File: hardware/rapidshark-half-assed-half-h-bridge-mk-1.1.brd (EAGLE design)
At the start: 17.8 x 33 mm, 29 parts, among them Q1 SPD15P10PL, Q2 IRLR3410, Q3 MMBT2222A, Q4 MMBT4403, U1 ARDUINO_PRO_MINIMINE

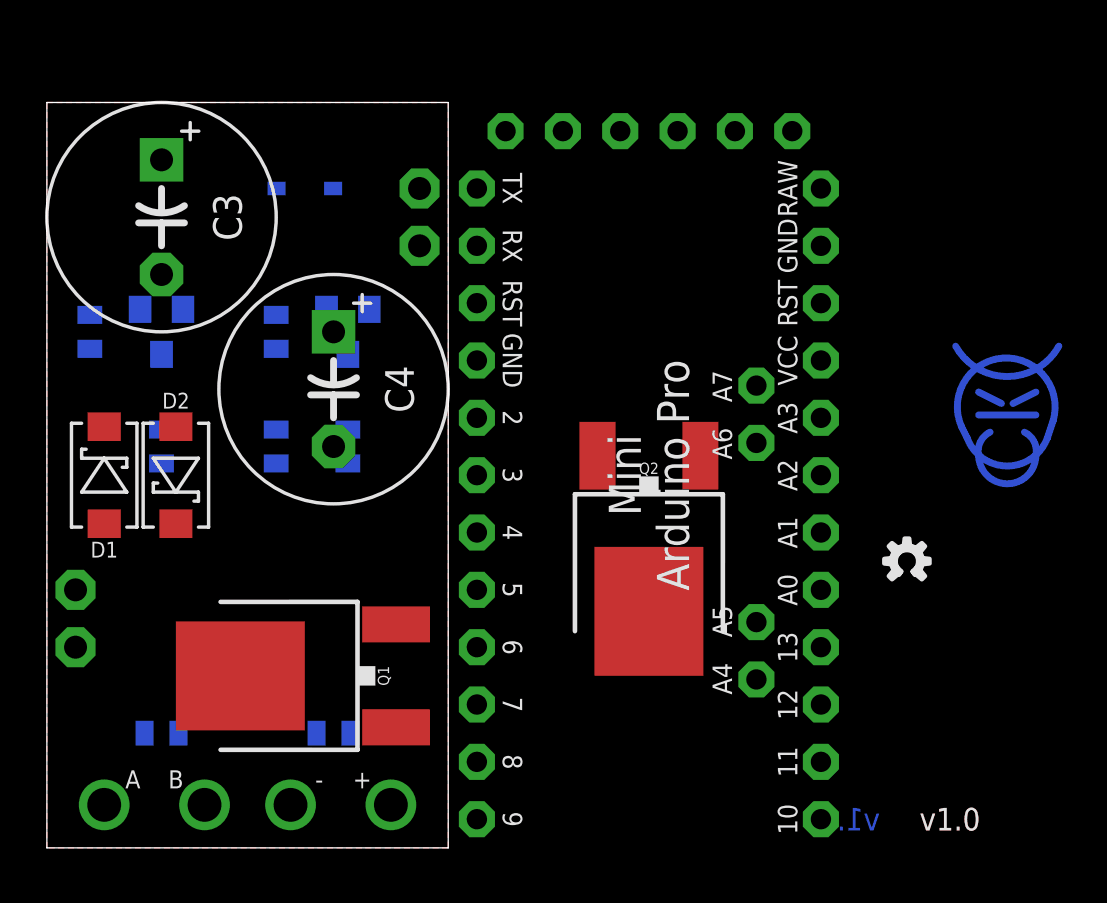
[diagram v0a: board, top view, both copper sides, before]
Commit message: more twiddling around with cheap h-bridge ideas
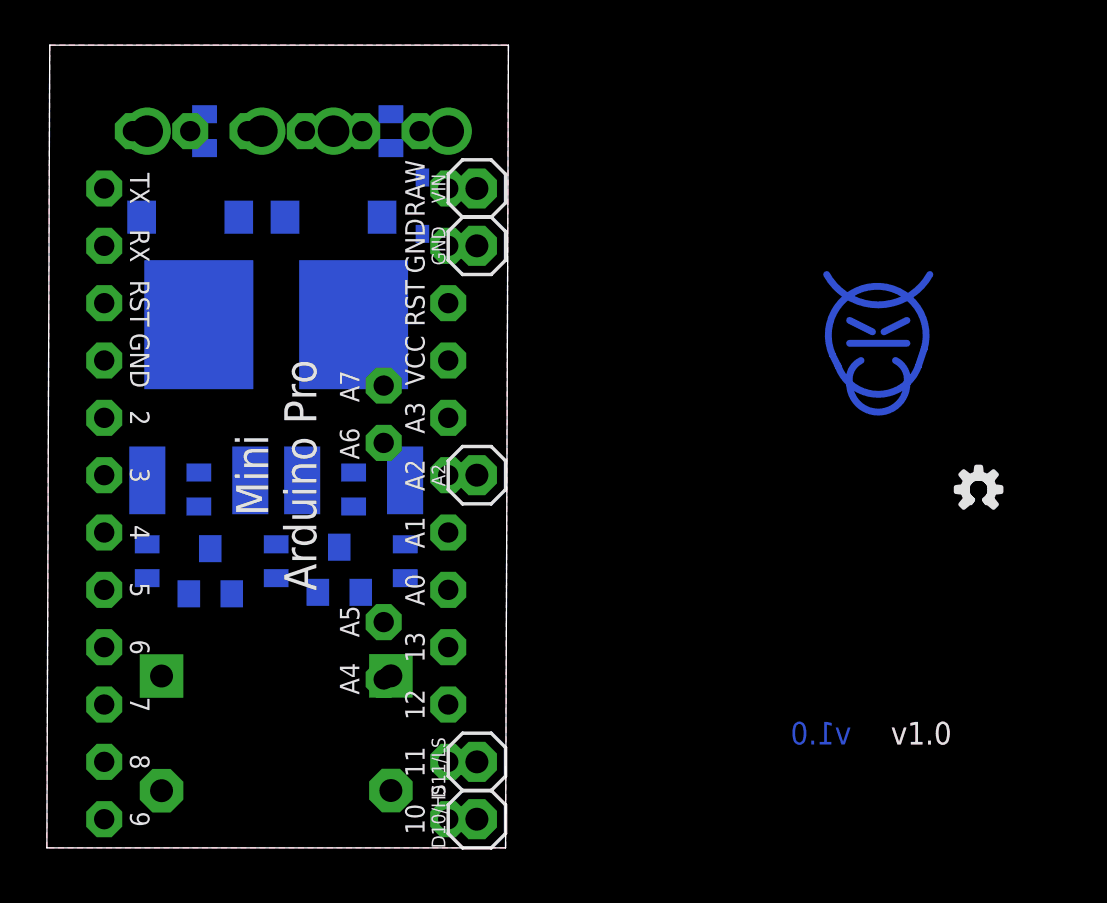
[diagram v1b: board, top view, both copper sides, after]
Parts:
- removed D5/HS, D6/LS: M01PTH, a_parts:1X01
- added A2, D10/HS, D11/LS: M01PTH, a_parts:1X01
- +, -, A, B: value M01PTH-1.5MM -> M01PTH-1.4MM; device a_parts:1X01-1.5MM-CIR -> a_parts:1X01-1.4MM-CIR
- moved + 30.0 mm to (17.8, 31.8), flipped to the bottom, turned to 0 degrees
- moved B 30.0 mm to (9.53, 31.8), flipped to the bottom, turned to 0 degrees
- moved A 29.9 mm to (4.45, 31.8), flipped to the bottom, turned to 0 degrees
- moved - 29.9 mm to (12.7, 31.8), flipped to the bottom, turned to 0 degrees
- moved C2 26.8 mm to (15.2, 31.8), turned to 90 degrees
- moved C1 26.7 mm to (6.99, 31.8), turned to 90 degrees
- moved C3 25.0 mm to (15.2, 5.08), flipped to the bottom
- moved Q2 22.1 mm to (6.73, 21.6), flipped to the bottom, turned to 0 degrees
- moved R3 17.3 mm to (15.9, 12.7)
- moved C4 17.0 mm to (5.08, 5.07), flipped to the bottom
- moved U1 16.5 mm to (10.2, 16.5)
- moved D1 15.3 mm to (12.7, 27.9), flipped to the bottom, turned to 180 degrees
- moved Q1 14.4 mm to (13.6, 21.6), flipped to the bottom, turned to 0 degrees
- moved Q3 13.2 mm to (13.0, 12.3), turned to 0 degrees
- moved Q4 12.2 mm to (7.24, 12.3), turned to 0 degrees
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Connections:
- removed net V_BATT: +.P$1, D1.C, Q1.3, R1.2
- net GND: no longer U1.23
- net HS: now also D10/HS.1; no longer D5/HS.1, U1.8
- net LS: now also D11/LS.1; no longer D6/LS.1, U1.9
- net VBAT: now also +.P$1, D1.C, Q1.3, R1.2; no longer U1.24
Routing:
- added copper zone on layer 16, net GND
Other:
- board size 17.8 x 33 mm -> 20.4 x 35.6 mm
